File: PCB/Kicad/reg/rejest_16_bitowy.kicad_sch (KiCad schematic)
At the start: 4 parts, among them U13 74AHCT374, U19 74AHCT374

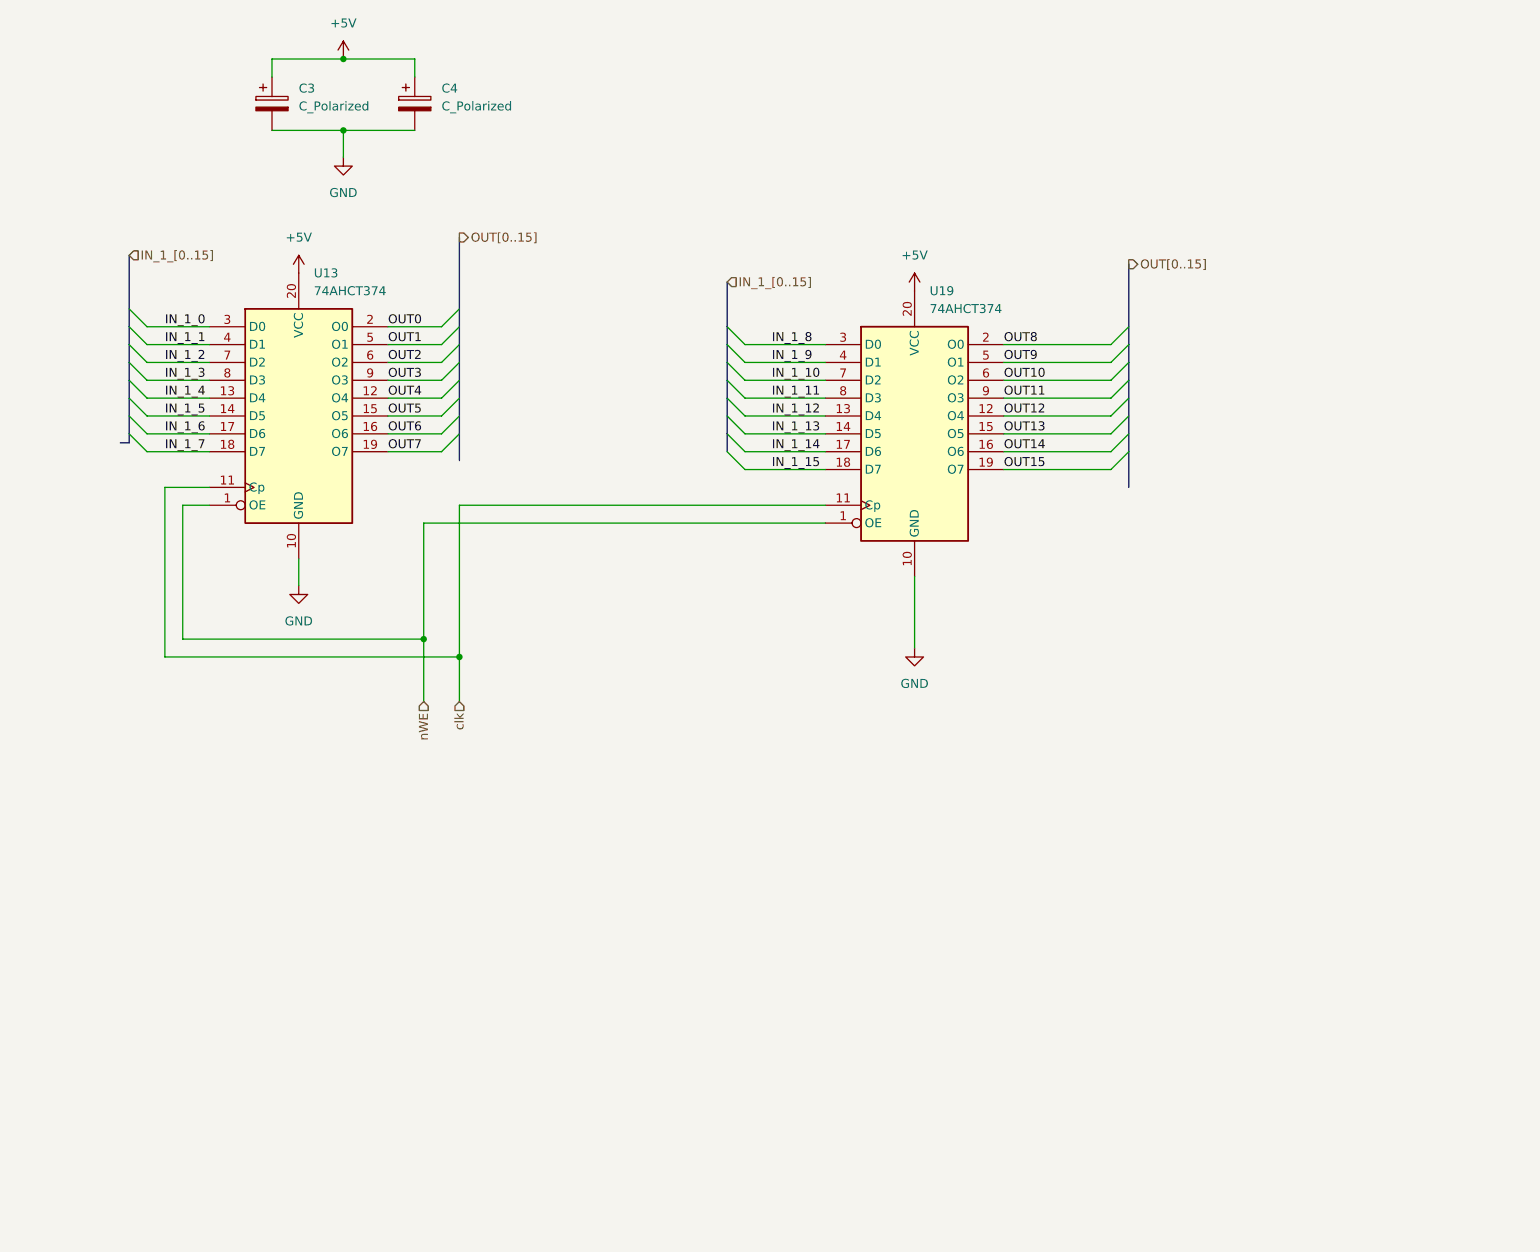
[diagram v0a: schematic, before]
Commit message: aaaaaaaaaaaaaaaaaaaaaaaaaaaaaaaaaaaaaaaaaaaa
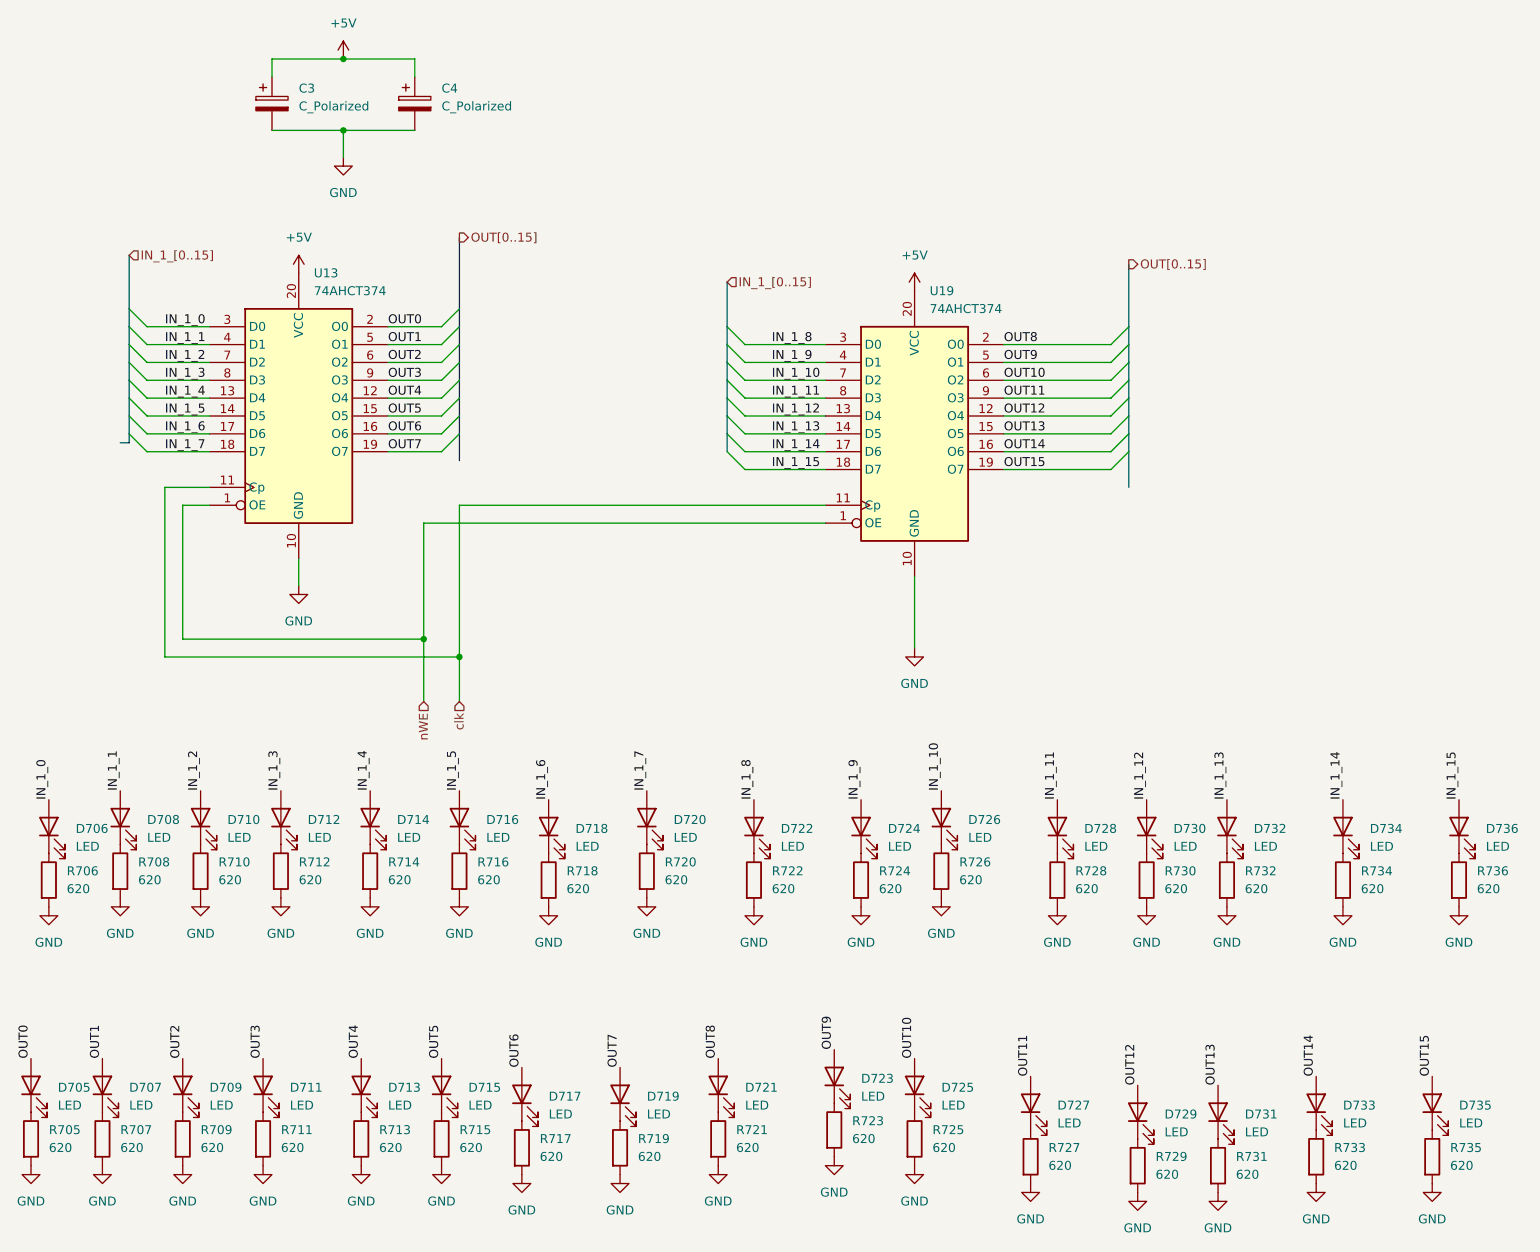
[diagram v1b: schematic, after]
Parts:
- added D705, D706, D707, D708, D709, D710, D711, D712, D713, D714, D715, D716, D717, D718, D719, D720, D721, D722, D723, D724, D725, D726, D727, D728, D729, D730, D731, D732, D733, D734, D735, D736: LED, LED_SMD:LED_0603_1608Metric_Pad1.05x0.95mm_HandSolder, symbol Device:LED
- added R705, R706, R707, R708, R709, R710, R711, R712, R713, R714, R715, R716, R717, R718, R719, R720, R721, R722, R723, R724, R725, R726, R727, R728, R729, R730, R731, R732, R733, R734, R735, R736: 620, Resistor_SMD:R_0402_1005Metric_Pad0.72x0.64mm_HandSolder, symbol Device:R
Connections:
- net GND: now also R705.2, R706.2, R707.2, R708.2, R709.2, R710.2, R711.2, R712.2, R713.2, R714.2, R715.2, R716.2, R717.2, R718.2, R719.2, R720.2, R721.2, R722.2, R723.2, R724.2, R725.2, R726.2, R727.2, R728.2, R729.2, R730.2, R731.2, R732.2, R733.2, R734.2, R735.2, R736.2
- net IN_1_0: now also D706.2 (A)
- net IN_1_1: now also D708.2 (A)
- net IN_1_10: now also D726.2 (A)
- net IN_1_11: now also D728.2 (A)
- net IN_1_12: now also D730.2 (A)
- net IN_1_13: now also D732.2 (A)
- net IN_1_14: now also D734.2 (A)
- net IN_1_15: now also D736.2 (A)
- net IN_1_2: now also D710.2 (A)
- net IN_1_3: now also D712.2 (A)
- net IN_1_4: now also D714.2 (A)
- net IN_1_5: now also D716.2 (A)
- net IN_1_6: now also D718.2 (A)
- net IN_1_7: now also D720.2 (A)
- net IN_1_8: now also D722.2 (A)
- net IN_1_9: now also D724.2 (A)
- net OUT0: now also D705.2 (A)
- net OUT1: now also D707.2 (A)
- net OUT10: now also D725.2 (A)
- net OUT11: now also D727.2 (A)
- net OUT12: now also D729.2 (A)
- net OUT13: now also D731.2 (A)
- net OUT14: now also D733.2 (A)
- net OUT15: now also D735.2 (A)
- net OUT2: now also D709.2 (A)
- net OUT3: now also D711.2 (A)
- net OUT4: now also D713.2 (A)
- net OUT5: now also D715.2 (A)
- net OUT6: now also D717.2 (A)
- net OUT7: now also D719.2 (A)
- net OUT8: now also D721.2 (A)
- net OUT9: now also D723.2 (A)
- new net: D727.1 (K), R727.1
- new net: D705.1 (K), R705.1
- new net: D734.1 (K), R734.1
- new net: D720.1 (K), R720.1
- new net: D733.1 (K), R733.1
- new net: D713.1 (K), R713.1
- new net: D729.1 (K), R729.1
- new net: D716.1 (K), R716.1
- new net: D728.1 (K), R728.1
- new net: D717.1 (K), R717.1
- new net: D722.1 (K), R722.1
- new net: D731.1 (K), R731.1
- new net: D706.1 (K), R706.1
- new net: D715.1 (K), R715.1
- new net: D719.1 (K), R719.1
- new net: D710.1 (K), R710.1
- new net: D732.1 (K), R732.1
- new net: D725.1 (K), R725.1
- new net: D735.1 (K), R735.1
- new net: D726.1 (K), R726.1
- new net: D712.1 (K), R712.1
- new net: D724.1 (K), R724.1
- new net: D709.1 (K), R709.1
- new net: D714.1 (K), R714.1
- new net: D708.1 (K), R708.1
- new net: D730.1 (K), R730.1
- new net: D736.1 (K), R736.1
- new net: D718.1 (K), R718.1
- new net: D711.1 (K), R711.1
- new net: D707.1 (K), R707.1
- new net: D721.1 (K), R721.1
- new net: D723.1 (K), R723.1
